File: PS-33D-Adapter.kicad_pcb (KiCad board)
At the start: 2 copper layers, 15 x 7.6 mm, 8 parts, among them J1 CONN_05, J2 Conn_02x04_Counter_Clockwise, Q1 MOSFET-NCH-BSS138, Q2 MOSFET-NCH-BSS138

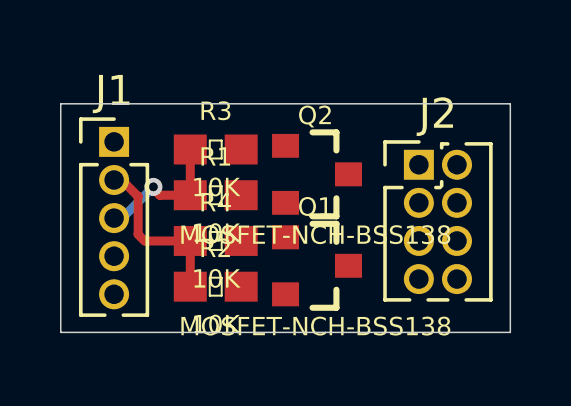
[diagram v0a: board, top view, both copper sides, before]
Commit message: feat: update schematic, pcb
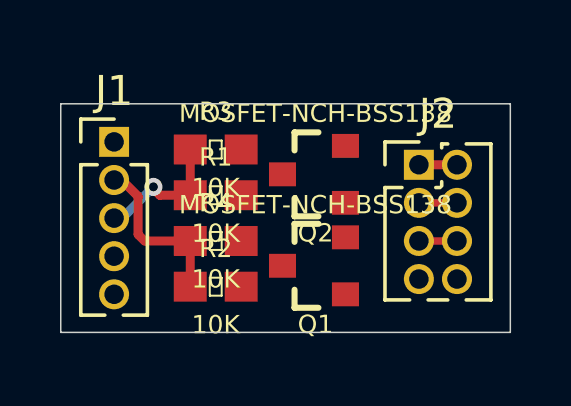
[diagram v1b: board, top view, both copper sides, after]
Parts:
- turned Q1 to 90 degrees
- turned Q2 to 90 degrees
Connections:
- J2 pad 2: SDA -> 3V3
- J2 pad 3: SCL -> SDA
- J2 pad 4: GND -> SDA
- J2 pad 5: GND -> SCL
- J2 pad 7: SDA -> GND
- J2 pad 8: 3V3 -> GND
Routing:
- net SDA: track 0.00 -> 1.27 mm
- net SCL: track 0.00 -> 1.27 mm
- net 3V3: track 4.65 -> 5.92 mm
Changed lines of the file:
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@@
     (thickness 1.6)
     (drawings 4)
-    (tracks 13)
+    (tracks 16)
     (zones 0)
     (modules 8)
@@
       (net 3 3V3))
     (pad 2 thru_hole oval (at 1.27 0) (size 1 1) (drill 0.65) (layers *.Cu *.Mask)
+      (net 3 3V3))
+    (pad 3 thru_hole oval (at 0 1.27) (size 1 1) (drill 0.65) (layers *.Cu *.Mask)
       (net 6 SDA))
-    (pad 3 thru_hole oval (at 0 1.27) (size 1 1) (drill 0.65) (layers *.Cu *.Mask)
+    (pad 4 thru_hole oval (at 1.27 1.27) (size 1 1) (drill 0.65) (layers *.Cu *.Mask)
+      (net 6 SDA))
+    (pad 5 thru_hole oval (at 0 2.54) (size 1 1) (drill 0.65) (layers *.Cu *.Mask)
       (net 7 SCL))
-    (pad 4 thru_hole oval (at 1.27 1.27) (size 1 1) (drill 0.65) (layers *.Cu *.Mask)
-      (net 1 GND))
-    (pad 5 thru_hole oval (at 0 2.54) (size 1 1) (drill 0.65) (layers *.Cu *.Mask)
-      (net 1 GND))
     (pad 6 thru_hole oval (at 1.27 2.54) (size 1 1) (drill 0.65) (layers *.Cu *.Mask)
       (net 7 SCL))
     (pad 7 thru_hole oval (at 0 3.81) (size 1 1) (drill 0.65) (layers *.Cu *.Mask)
-      (net 6 SDA))
+      (net 1 GND))
     (pad 8 thru_hole oval (at 1.27 3.81) (size 1 1) (drill 0.65) (layers *.Cu *.Mask)
-      (net 3 3V3))
+      (net 1 GND))
     (model ${KISYS3DMOD}/Connector_PinHeader_1.27mm.3dshapes/PinHeader_2x04_P1.27mm_Vertical.wrl
       (at (xyz 0 0 0))
@@
   )
   (module Silicon-Standard:SOT23-3 (layer F.Cu)
-    (at 154.03322 82.87004 270)
+    (at 154.03322 82.87004 90)
     (descr SOT23-3)
     (tags SOT23-3)
@@
     (fp_line (start 0.79756 -0.6985) (end 1.39954 -0.6985) (layer F.SilkS) (width 0.2032))
     (fp_line (start 1.39954 -0.6985) (end 1.39954 0.09906) (layer F.SilkS) (width 0.2032))
-    (pad 1 smd rect (at -0.94996 0.99822 270) (size 0.79756 0.89916) (layers F.Cu F.Paste F.Mask)
+    (pad 1 smd rect (at -0.94996 0.99822 90) (size 0.79756 0.89916) (layers F.Cu F.Paste F.Mask)
       (net 3 3V3) (solder_mask_margin 0.1016))
-    (pad 2 smd rect (at 0.94996 0.99822 270) (size 0.79756 0.89916) (layers F.Cu F.Paste F.Mask)
+    (pad 2 smd rect (at 0.94996 0.99822 90) (size 0.79756 0.89916) (layers F.Cu F.Paste F.Mask)
       (net 6 SDA) (solder_mask_margin 0.1016))
-    (pad 3 smd rect (at 0 -1.09982 270) (size 0.79756 0.89916) (layers F.Cu F.Paste F.Mask)
+    (pad 3 smd rect (at 0 -1.09982 90) (size 0.79756 0.89916) (layers F.Cu F.Paste F.Mask)
       (net 5 M.SDA) (solder_mask_margin 0.1016))
   )
   (module Silicon-Standard:SOT23-3 (layer F.Cu)
-    (at 154.03322 79.82204 270)
+    (at 154.03322 79.82204 90)
     (descr SOT23-3)
     (tags SOT23-3)
@@
     (fp_line (start 1.4224 0.6604) (end -1.4224 0.6604) (layer Dwgs.User) (width 0.1524))
     (fp_line (start 1.4224 -0.6604) (end 1.4224 0.6604) (layer Dwgs.User) (width 0.1524))
-    (pad 3 smd rect (at 0 -1.09982 270) (size 0.79756 0.89916) (layers F.Cu F.Paste F.Mask)
+    (pad 3 smd rect (at 0 -1.09982 90) (size 0.79756 0.89916) (layers F.Cu F.Paste F.Mask)
       (net 4 M.SCL) (solder_mask_margin 0.1016))
-    (pad 2 smd rect (at 0.94996 0.99822 270) (size 0.79756 0.89916) (layers F.Cu F.Paste F.Mask)
+    (pad 2 smd rect (at 0.94996 0.99822 90) (size 0.79756 0.89916) (layers F.Cu F.Paste F.Mask)
       (net 7 SCL) (solder_mask_margin 0.1016))
-    (pad 1 smd rect (at -0.94996 0.99822 270) (size 0.79756 0.89916) (layers F.Cu F.Paste F.Mask)
+    (pad 1 smd rect (at -0.94996 0.99822 90) (size 0.79756 0.89916) (layers F.Cu F.Paste F.Mask)
       (net 3 3V3) (solder_mask_margin 0.1016))
   )
@@
   (segment (start 148.629651 80.303651) (end 148.844 80.518) (width 0.3) (layer F.Cu) (net 3))
   (segment (start 149.86 80.518) (end 149.86 78.994) (width 0.3) (layer F.Cu) (net 3))
+  (segment (start 157.48 79.502) (end 158.75 79.502) (width 0.3) (layer F.Cu) (net 3))
+  (segment (start 157.48 80.772) (end 158.75 80.772) (width 0.25) (layer F.Cu) (net 6))
+  (segment (start 157.48 82.042) (end 158.75 82.042) (width 0.25) (layer F.Cu) (net 7))
 )
